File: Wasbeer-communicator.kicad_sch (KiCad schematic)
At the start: 20 parts, among them IC1 E22-900M22S, Q1 DMG2302U, SW1 SW_Push, U1 TP4056, U2 Pico

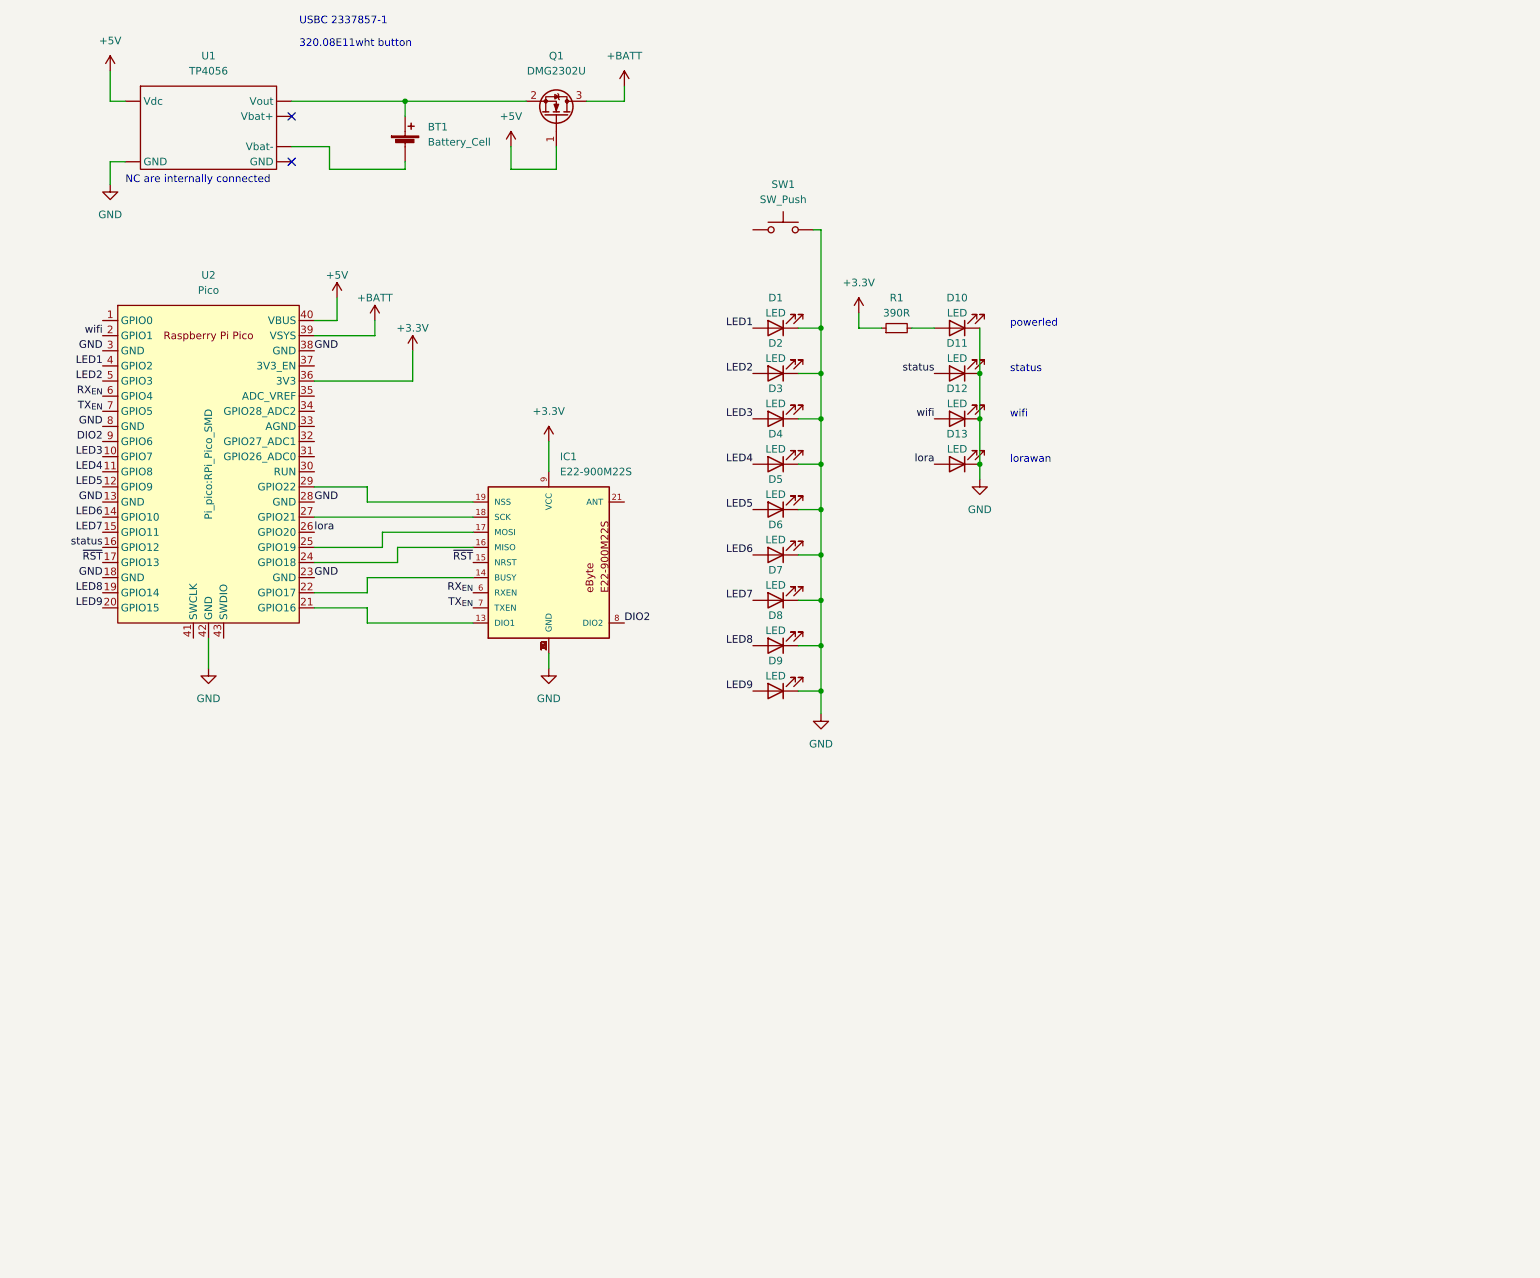
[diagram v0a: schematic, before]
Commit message: Finished design, created gerbers for lcsc
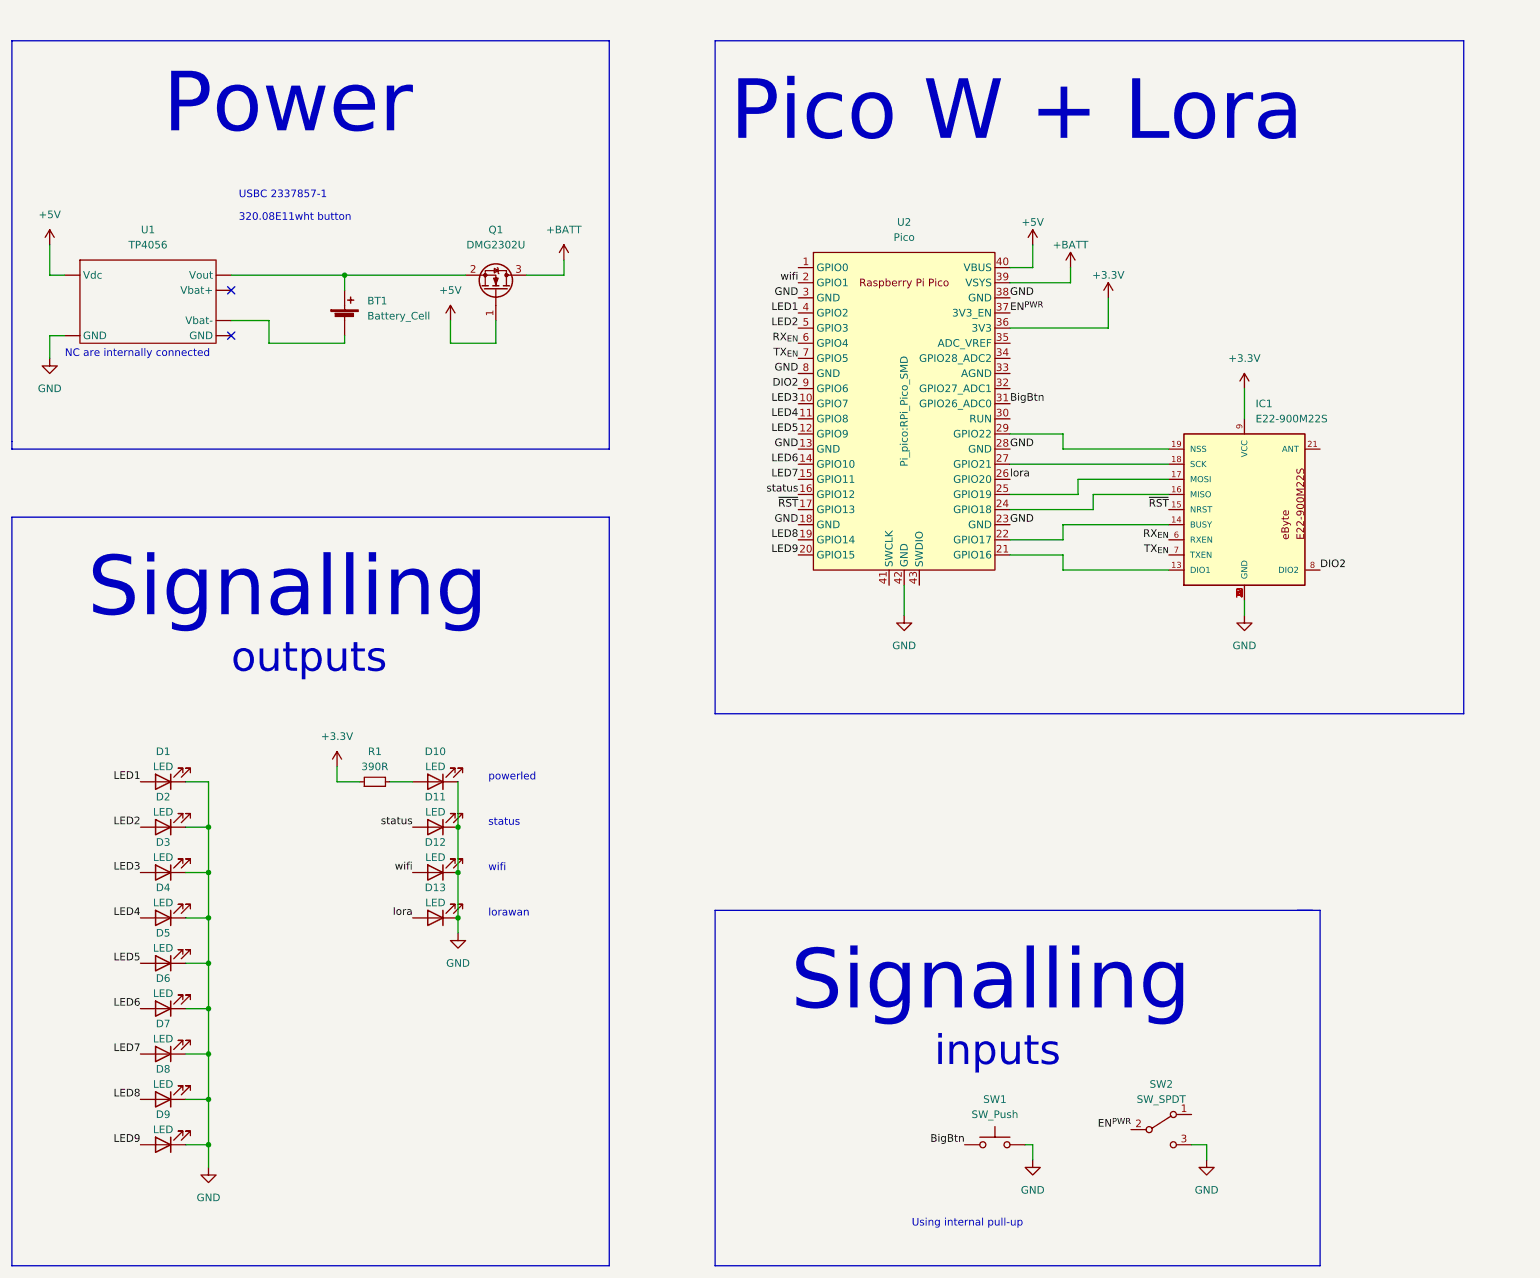
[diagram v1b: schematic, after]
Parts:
- added SW2: SW_SPDT, Pi_pico:MSS3-Q-TR, symbol Switch:SW_SPDT
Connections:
- net GND: now also SW2.3 (C)
- net BigBtn: now reaches SW1.1
- net BigBtn: now also U2.31 (GPIO26_ADC0)
- net EN^{PWR}: now reaches U2.37 (3V3_EN)
- net EN^{PWR}: now also SW2.2 (B)
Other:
- note added: "Pico W + Lora"
- note added: "Power"
- note added: "Signalling"
- note added: "Using internal pull-up"
- note added: "inputs"
- note added: "outputs"
- moved on the sheet: BT1, D1, D10, D11, D12, D13, D2, D3, D4, D5, D6, D7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
